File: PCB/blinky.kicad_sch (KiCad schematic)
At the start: 1 part, among them U1 7555

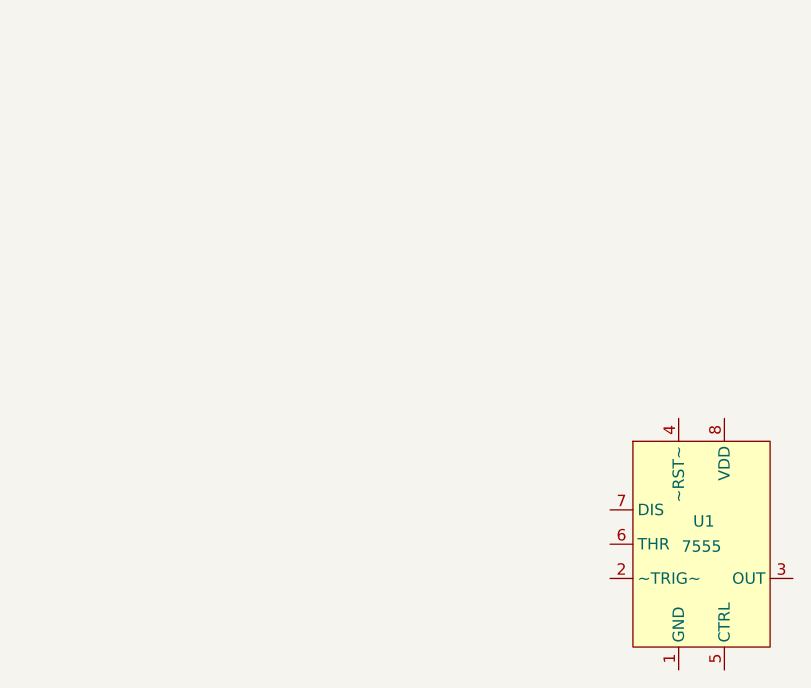
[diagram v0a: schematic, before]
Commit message: Create schematic
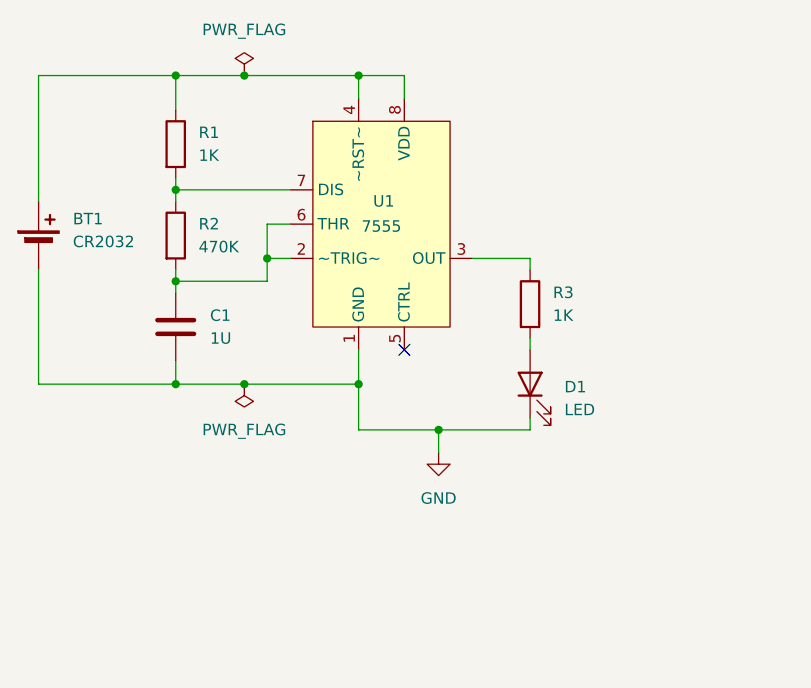
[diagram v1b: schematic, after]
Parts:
- added BT1: CR2032, symbol Device:Battery_Cell
- added C1: 1U, symbol Device:C
- added D1: LED, symbol Device:LED
- added R1, R3: 1K, symbol Device:R
- added R2: 470K, symbol Device:R
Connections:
- net GND: now reaches U1.1 (GND)
- net GND: now also BT1.2 (-), C1.2, D1.1 (K)
- net at U1.2 (~TRIG~): now also U1.6 (THR), C1.1, R2.2
- net at U1.3 (OUT): now also R3.1
- net at U1.4 (~RST~): now also U1.8 (VDD), BT1.1 (+), R1.1
- net at U1.7 (DIS): now also R1.2, R2.1
- new net: D1.2 (A), R3.2
- no-connect marks 0 -> 1
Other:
- moved on the sheet: U1
